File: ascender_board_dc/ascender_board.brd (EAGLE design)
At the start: 94 x 80 mm, 46 parts, among them IC1 LM2937, IC2 MC33932, Q1 8MHz, U1 STM32F722XX, X1 MINI-USB-32005-201, X2 52745-1890, X3 52745-1890

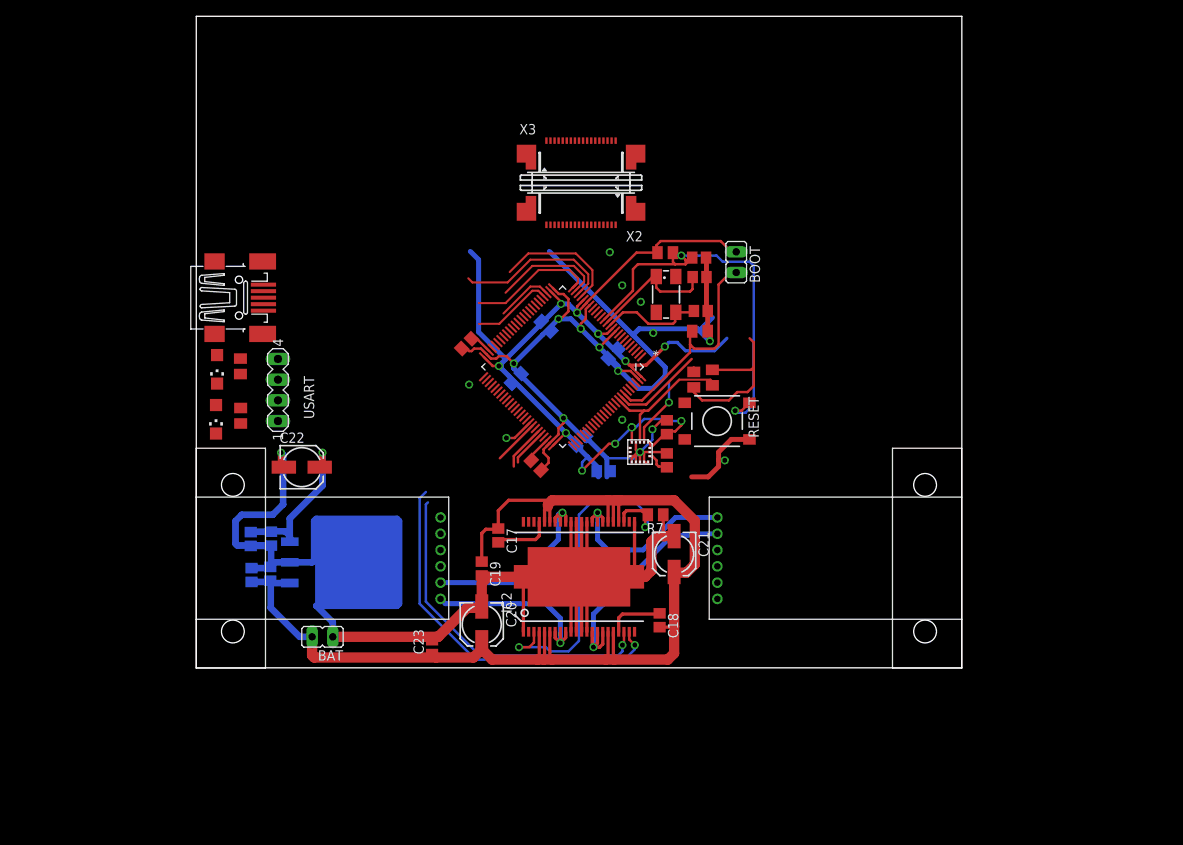
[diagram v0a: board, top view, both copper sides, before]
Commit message: board
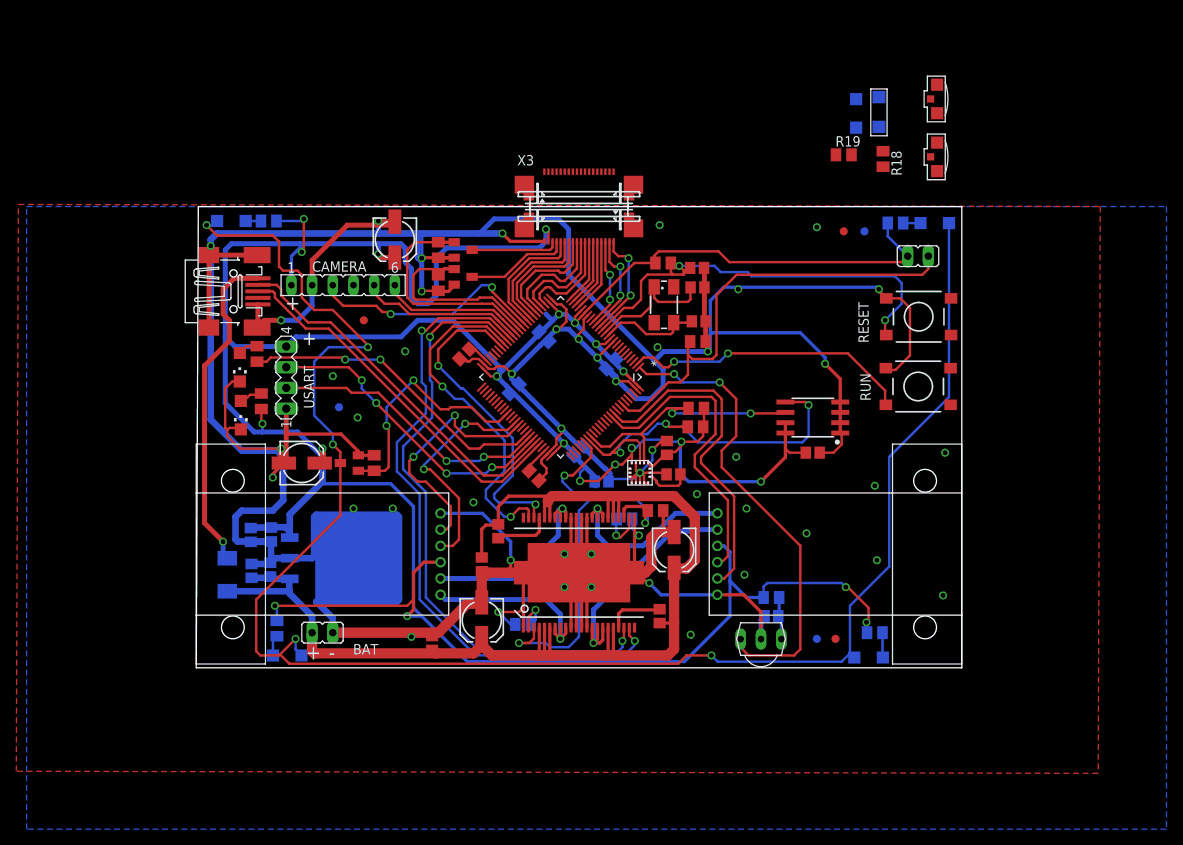
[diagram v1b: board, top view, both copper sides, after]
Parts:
- removed X1: MINI-USB-32005-201, con-cypressindustries:32005-201
- added C24: (no value), resistor:153CLV-0505
- added C25: 10uF, resistor:C0805
- added C26: 100n, resistor:C0805
- added CAMERA: (no value), con-lsta:FE06
- added D1: (no value), diode:DO-214AC
- added LED3, LED4, LED5, LED6, LED7: (no value), my_parts:CHIPLED_1206
- added Q2, Q3, Q4: BSS123, transistor-small-signal:SOT23
- added R10, R11, R12, R18, R8, R9: 4k7, resistor:M0805
- added R13, R14, R15, R16, R19: 330, resistor:M0805
- added R17: 22, resistor:M0805
- added RUN: DTSM-6, switch-tact:DTSM-6
- added U$11: SFH3710, my_parts:SFH3710
- added U$12: KPA3010, my_parts:KPA3010
- added U$13: KPA3010_EM, my_parts:KPA3010
- added U$3, U$4, U$5, U$6, U$7, U$8: FIDUCIAL, adafruit:FIDUCIAL_1MM
- added U$9: TSOP4830, tsop:TSOP18XX
- added U2: I2C EEPROM, SparkFun-IC-Memory:SO08-EIAJ
- added X4: MINI-USB-SCHIELD-32005-201, con-cypressindustries:32005-201
- moved RESET 27.9 mm to (88.7, 43.1), turned to 0 degrees
- moved BOOT 22.3 mm to (88.6, 50.6), turned to 90 degrees
- moved R4 6.39 mm to (61.3, 29.6), turned to 0 degrees
- moved X3 3.82 mm to (47.0, 58.4)
- moved R5 3.52 mm to (61.4, 31.9), turned to 0 degrees
- moved R6 3.10 mm to (7.99, 32.7)
- moved LED2 3.09 mm to (5.47, 31.0)
- moved LED1 2.81 mm to (5.35, 36.9)
- moved C15 2.54 mm to (57.8, 27.0)
- moved R3 2.54 mm to (7.46, 38.5)
- moved U$2 2.54 mm to (54.5, 24.0)
- moved X2 2.05 mm to (47.0, 54.9)
- moved C14 1.91 mm to (58.6, 23.7), turned to 180 degrees
- moved USART 1.83 mm to (11.0, 35.6)
- moved C4 1.30 mm to (32.9, 38.5)
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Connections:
- removed net +5V: X1.1
- new net ADC10: U1.34, X2.14
- new net ADC11: CAMERA.3, U1.35
- new net ADC1_S: R18.1, U$11.P$2, X3.14
- new net CAM_CLK: CAMERA.5, U1.39
- new net CAM_SI: CAMERA.6, U1.38
- new net FRONT_SCL: U1.15, X2.1
- new net FRONT_SDA: U1.16, X2.2
- new net IR_A: Q2.3, X2.15
- new net IR_A_CONTROLL: Q2.1, R10.2, U1.36
- new net IR_A_S: R19.1, X3.4
- new net IR_B: Q3.3, X2.16
- new net IR_B_CONTROLL: Q3.1, R11.2, U1.37
- new net IR_REMOTE: U$9.OUT, U1.1
- new net LED_BACK: Q4.1, R12.2, U1.60
- new net N$13: IC2.2, R8.2
- new net N$15: IC2.24, R9.1
- new net N$16: LED3.C, LED4.C, LED5.C, LED6.C, Q4.3
- new net N$17: LED3.A, R13.1
- new net N$18: D1.A, X4.1
- new net N$19: LED4.A, R14.1
- new net N$20: C25.1, R17.1, U$9.VCC
- new net N$21: LED5.A, R15.1
- new net N$23: LED6.A, R16.1
- new net N$24: LED7.C, R19.2
- new net NC: CAMERA.4
- net +3V3: now also C24.+, C26.1, CAMERA.1, LED7.A, R13.2, R14.2, R15.2, R16.2, R17.2, R18.2, U2.7, U2.8, X2.17, X3.2; no longer X2.18
- net ADC0: now also X2.4
- net ADC1: now also X2.5
- net ADC2: now also X2.6
- net ADC3: now also X2.7
- net ADC4: now also X2.8
- net ADC5: now also X2.9
- net ADC6: now also X2.10
- net ADC7: now also X2.11
- net ADC8: now also U1.32, X2.12; no longer U1.34
- net ADC9: now also U1.33, X2.13; no longer U1.35
- net ENC_A_LEFT: now also U1.63; no longer U1.2
- net ENC_A_RIGHT: now also U1.90; no longer U1.4
- net ENC_B_LEFT: now also U1.64; no longer U1.3
- net ENC_B_RIGHT: now also U1.91; no longer U1.5
- net FRONT_GPIO: now also U1.17
- net GND: now also C24.-, C25.2, C26.2, CAMERA.2, Q2.2, Q3.2, Q4.2, R10.1, R11.1, R12.1, R8.1, R9.2, RUN.1, U$11.P$1, U$9.GND, U2.1, U2.2, U2.3, U2.4, X2.18, X3.1, X4.5, X4.M1, X4.M2, X4.M3, X4.M4; no longer X1.5, X2.17
- net KEY: now also RUN.3, U1.2; no longer U1.66
- net MOTOR_ENABLE: now also U1.81; no longer U1.44
- net SCL: now also U1.83, U2.6; no longer U1.93, X2.1
- net SDA: now also U1.82, U2.5; no longer U1.92, X2.2
- net USBDM: now also X4.2; no longer X1.2
- net USBDP: now also X4.3; no longer X1.3
- net VCC: now also D1.C
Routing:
- net GND: track 359.1 -> 659.2 mm, vias 17 -> 48
- net +3V3: track 179.5 -> 470.3 mm, vias 13 -> 22
- net N$16: track 0.00 -> 219.8 mm, vias 0 -> 5
- net IR_REMOTE: track 0.00 -> 58.0 mm, vias 0 -> 2
- net PWM_A_LEFT: track 0.00 -> 42.5 mm, vias 0 -> 2
- net ENC_B_RIGHT: track 0.00 -> 41.8 mm
- net USBDP: track 4.63 -> 46.4 mm
- net N$18: track 0.00 -> 40.6 mm, vias 0 -> 1
- net USBDM: track 5.55 -> 46.0 mm
- net PWM_B_LEFT: track 0.00 -> 39.8 mm, vias 0 -> 2
- net ENC_A_RIGHT: track 0.00 -> 38.6 mm
- net USART1_RX: track 0.00 -> 38.1 mm, vias 0 -> 4
- net KEY: track 0.00 -> 35.7 mm, vias 0 -> 2
- net LED: track 3.85 -> 38.9 mm, vias 1 -> 2
- net PWM_A_RIGHT: track 46.2 -> 80.6 mm, vias 1 -> 2
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- added copper zone on layer 1, net GND
- added copper zone on layer 16, net GND
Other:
- board size 94 x 80 mm -> 94 x 56.6 mm
- board text added: "+"
- board text added: "-"
